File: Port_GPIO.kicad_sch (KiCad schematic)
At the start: 16 parts, among them J1 Conn_01x03_Pin, J10 Conn_01x06_Pin, J11 Conn_01x05_Pin, J2 Conn_01x03_Pin, J3 USB_C_Receptacle_USB2.0_14P, J4 Conn_01x06_Pin, J5 TC2030, J8 Conn_01x05_Pin, J9 Conn_01x06_Pin, U2 USBLC6-2SC6

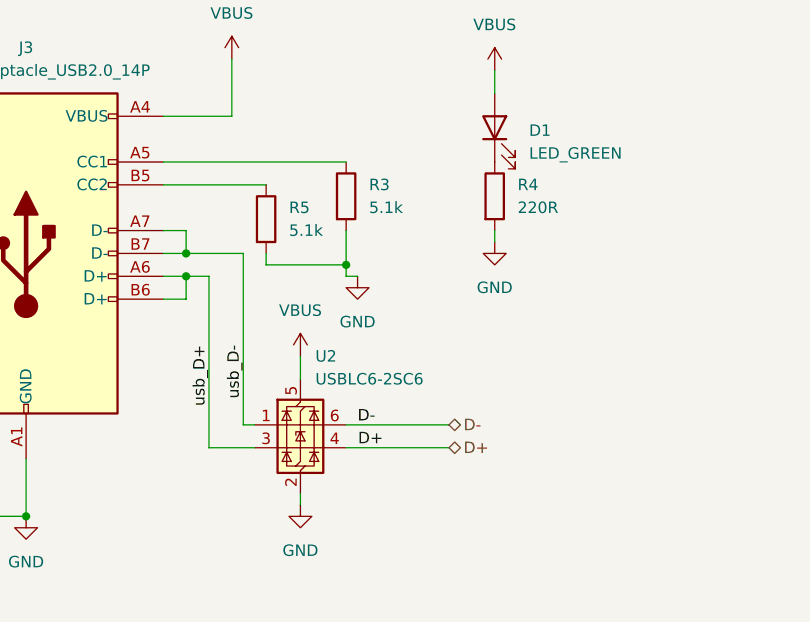
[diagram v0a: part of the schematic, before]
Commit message: Updatte
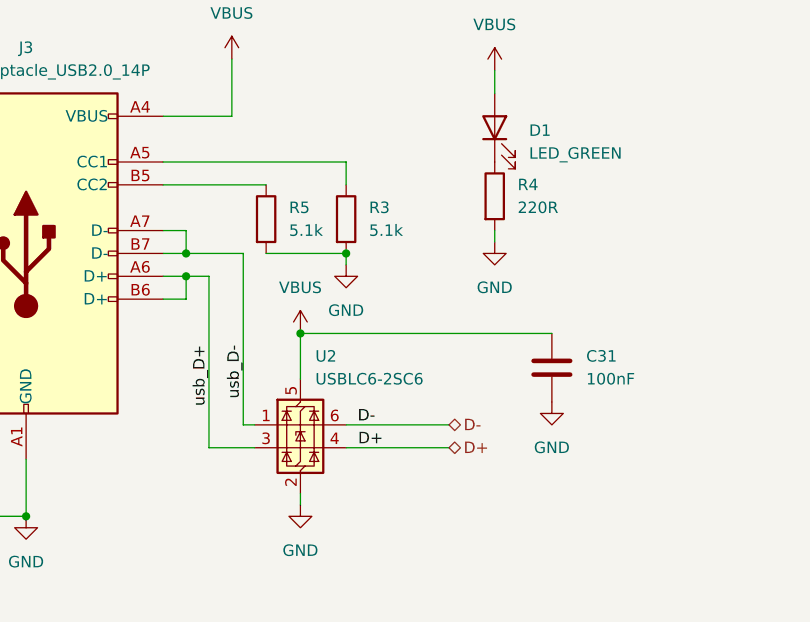
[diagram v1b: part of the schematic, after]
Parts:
- added C31: 100nF, Capacitor_SMD:C_0603_1608Metric_Pad1.08x0.95mm_HandSolder, symbol Device:C
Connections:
- net GND: now also C31.2
- net VBUS: now also C31.1
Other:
- moved on the sheet: R3
